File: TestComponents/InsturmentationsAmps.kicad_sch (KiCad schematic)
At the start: 42 parts, among them SW2 SW_DP3T, SW3 SW_DPDT, U3 REF200AU, U4 MCP6L01x-xLT

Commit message: SpectDrone Development
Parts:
- CS1, CS6: footprint Capacitor_SMD:C_0805_2012Metric -> Capacitor_SMD:C_0603_1608Metric; Part Number (none) -> 06035J100FBTTR
- CS2, CS3, CS7, CS8: footprint Capacitor_SMD:C_0805_2012Metric -> Capacitor_SMD:C_0402_1005Metric; Part Number (none) -> 04023J1R1PBSTR
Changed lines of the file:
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@@
       (effects (font (size 1.27 1.27)) (justify left))
     )
-    (property "Footprint" "Capacitor_SMD:C_0805_2012Metric" (id 2) (at 217.17 44.45 0)
+    (property "Footprint" "Capacitor_SMD:C_0402_1005Metric" (id 2) (at 217.17 44.45 0)
       (effects (font (size 1.27 1.27)) hide)
     )
     (property "Datasheet" "~" (id 3) (at 217.17 44.45 0)
+      (effects (font (size 1.27 1.27)) hide)
+    )
+    (property "Part Number" "04023J1R1PBSTR" (id 4) (at 217.17 44.45 0)
       (effects (font (size 1.27 1.27)) hide)
     )
@@
       (effects (font (size 1.27 1.27)) (justify left))
     )
-    (property "Footprint" "Capacitor_SMD:C_0805_2012Metric" (id 2) (at 214.63 54.61 0)
+    (property "Footprint" "Capacitor_SMD:C_0603_1608Metric" (id 2) (at 214.63 54.61 0)
       (effects (font (size 1.27 1.27)) hide)
     )
     (property "Datasheet" "~" (id 3) (at 214.63 54.61 0)
+      (effects (font (size 1.27 1.27)) hide)
+    )
+    (property "Part Number" "06035J100FBTTR" (id 4) (at 214.63 54.61 0)
       (effects (font (size 1.27 1.27)) hide)
     )
@@
       (effects (font (size 1.27 1.27)) (justify left))
     )
-    (property "Footprint" "Capacitor_SMD:C_0805_2012Metric" (id 2) (at 214.63 85.09 0)
+    (property "Footprint" "Capacitor_SMD:C_0603_1608Metric" (id 2) (at 214.63 85.09 0)
       (effects (font (size 1.27 1.27)) hide)
     )
     (property "Datasheet" "~" (id 3) (at 214.63 85.09 0)
+      (effects (font (size 1.27 1.27)) hide)
+    )
+    (property "Part Number" "06035J100FBTTR" (id 4) (at 214.63 85.09 0)
       (effects (font (size 1.27 1.27)) hide)
     )
@@
       (effects (font (size 1.27 1.27)) (justify left))
     )
-    (property "Footprint" "Capacitor_SMD:C_0805_2012Metric" (id 2) (at 214.63 95.25 0)
+    (property "Footprint" "Capacitor_SMD:C_0402_1005Metric" (id 2) (at 214.63 95.25 0)
       (effects (font (size 1.27 1.27)) hide)
     )
@@
       (effects (font (size 1.27 1.27)) hide)
     )
+    (property "Part Number" "04023J1R1PBSTR" (id 4) (at 214.63 95.25 0)
+      (effects (font (size 1.27 1.27)) hide)
+    )
     (pin "1")
     (pin "2")
@@
       (effects (font (size 1.27 1.27)) (justify left))
     )
-    (property "Footprint" "Capacitor_SMD:C_0805_2012Metric" (id 2) (at 214.63 64.77 0)
+    (property "Footprint" "Capacitor_SMD:C_0402_1005Metric" (id 2) (at 214.63 64.77 0)
       (effects (font (size 1.27 1.27)) hide)
     )
@@
       (effects (font (size 1.27 1.27)) hide)
     )
+    (property "Part Number" "04023J1R1PBSTR" (id 4) (at 214.63 64.77 0)
+      (effects (font (size 1.27 1.27)) hide)
+    )
     (pin "1")
     (pin "2")
@@
       (effects (font (size 1.27 1.27)) (justify left))
     )
-    (property "Footprint" "Capacitor_SMD:C_0805_2012Metric" (id 2) (at 217.17 74.93 0)
+    (property "Footprint" "Capacitor_SMD:C_0402_1005Metric" (id 2) (at 217.17 74.93 0)
       (effects (font (size 1.27 1.27)) hide)
     )
@@
       (effects (font (size 1.27 1.27)) hide)
     )
+    (property "Part Number" "04023J1R1PBSTR" (id 4) (at 217.17 74.93 0)
+      (effects (font (size 1.27 1.27)) hide)
+    )

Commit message: SpectDrone Development
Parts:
- CS10, CS11, CS13, CS5: Part Number (none) -> CL21B104KACNNNC
- CS12, CS4, CS9: Part Number (none) -> CL21A106KACLRNC
- JPD1, JPD2, JPD3, JPD4, JPD5, JPD6, PD1, PD2: now left out of the parts list
- R1: Part Number (none) -> ERA-6VRW1002V
- R2: Part Number (none) -> ERJ-PB6B2671V
- RS3, RS6, RS7, RS8: Part Number (none) -> ERA-6VEB3300V
- R_{C}1: Part Number (none) -> ERJ-PB6B4990V
- R_{PD.bias}1, R_{PD.bias}2: Part Number (none) -> ERJ-6GEY0R00V
- R_{PD}1, R_{PD}2: Part Number (none) -> ERA-6AEB105V
- R_{PD}1.1, R_{PD}2.1: Part Number (none) -> ERJ-6ENF2001V
- SW2: Part Number (none) -> JS203011JAQN
- SW3: Part Number (none) -> JS202011JAQN
- U3: Part Number (none) -> REF200AU
- U4: Part Number (none) -> MCP6L01T-E/LT
- US1, US2: Part Number (none) -> AD8221ARMZ
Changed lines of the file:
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@@
+      (effects (font (size 1.27 1.27)) hide)
+    )
+    (property "Part Number" "ERJ-6ENF2001V" (id 4) (at 195.58 80.01 0)
       (effects (font (size 1.27 1.27)) hide)
     )
@@
     )
     (property "Datasheet" "~" (id 3) (at 243.84 67.31 0)
+      (effects (font (size 1.27 1.27)) hide)
+    )
+    (property "Part Number" "CL21B104KACNNNC" (id 4) (at 243.84 67.31 0)
       (effects (font (size 1.27 1.27)) hide)
     )
@@
     )
     (property "Datasheet" "https://www.analog.com/media/en/technical-documentation/data-sheets/AD8236.pdf" (id 3) (at 248.92 44.45 0)
+      (effects (font (size 1.27 1.27)) hide)
+    )
+    (property "Part Number" "AD8221ARMZ" (id 4) (at 240.03 54.61 0)
       (effects (font (size 1.27 1.27)) hide)
     )
@@
       (effects (font (size 1.27 1.27)) hide)
     )
+    (property "Part Number" "ERA-6VEB3300V" (id 4) (at 208.28 59.69 0)
+      (effects (font (size 1.27 1.27)) hide)
+    )
     (pin "1")
     (pin "2")
@@
       (effects (font (size 1.27 1.27)) hide)
     )
+    (property "Part Number" "ERA-6VRW1002V" (id 4) (at 62.23 98.425 0)
+      (effects (font (size 1.27 1.27)) hide)
+    )
     (pin "1")
     (pin "2")
@@
     )
     (property "Datasheet" "~" (id 3) (at 200.025 54.61 0)
+      (effects (font (size 1.27 1.27)) hide)
+    )
+    (property "Part Number" "ERA-6AEB105V" (id 4) (at 200.025 54.61 0)
       (effects (font (size 1.27 1.27)) hide)
     )
@@
     )
     (property "Datasheet" "https://www.analog.com/media/en/technical-documentation/data-sheets/AD8236.pdf" (id 3) (at 248.92 74.93 0)
+      (effects (font (size 1.27 1.27)) hide)
+    )
+    (property "Part Number" "AD8221ARMZ" (id 4) (at 240.03 85.09 0)
       (effects (font (size 1.27 1.27)) hide)
     )
@@
       (effects (font (size 1.27 1.27)) hide)
     )
+    (property "Part Number" "ERJ-PB6B4990V" (id 4) (at 125.73 57.15 0)
+      (effects (font (size 1.27 1.27)) hide)
+    )
     (pin "1")
     (pin "2")
   )
   (symbol (lib_id "Jumper:SolderJumper_2_Bridged") (at 194.945 59.69 0) (unit 1)
-    (in_bom yes) (on_board yes)
+    (in_bom no) (on_board yes)
     (property "Reference" "JPD3" (id 0) (at 194.945 62.23 0))
     (property "Value" "SolderJumper_2_Bridged" (id 1) (at 201.295 62.23 0)
@@
     )
     (property "Datasheet" "~" (id 3) (at 208.28 90.17 0)
+      (effects (font (size 1.27 1.27)) hide)
+    )
+    (property "Part Number" "ERA-6VEB3300V" (id 4) (at 208.28 90.17 0)
       (effects (font (size 1.27 1.27)) hide)
     )
@@
     (property "Datasheet" "www.ti.com/lit/ds/symlink/ref200.pdf" (id 3) (at 64.135 71.755 0)
       (effects (font (size 1.27 1.27) italic) hide)
+    )
+    (property "Part Number" "REF200AU" (id 4) (at 71.755 71.755 0)
+      (effects (font (size 1.27 1.27)) hide)
     )
     (pin "6")
@@
       (effects (font (size 1.27 1.27)) hide)
     )
+    (property "Part Number" "JS203011JAQN" (id 4) (at 152.4 46.99 0)
+      (effects (font (size 1.27 1.27)) hide)
+    )
     (pin "1")
     (pin "2")
@@
   )
   (symbol (lib_id "Sensor_Optical:S13360-3025CS") (at 182.88 54.61 270) (unit 1)
-    (in_bom yes) (on_board yes)
+    (in_bom no) (on_board yes)
     (property "Reference" "PD1" (id 0) (at 179.07 53.34 90))
     (property "Value" "S1336-18BK" (id 1) (at 173.99 55.88 90))
@@
   )
   (symbol (lib_id "Jumper:SolderJumper_2_Bridged") (at 186.69 80.01 0) (unit 1)
-    (in_bom yes) (on_board yes)
+    (in_bom no) (on_board yes)
     (property "Reference" "JPD4" (id 0) (at 186.69 82.55 0))
     (property "Value" "SolderJumper_2_Bridged" (id 1) (at 193.04 82.55 0)
@@
       (effects (font (size 1.27 1.27) italic) hide)
     )
+    (property "Part Number" "REF200AU" (id 4) (at 68.58 52.705 0)
+      (effects (font (size 1.27 1.27)) hide)
+    )
     (pin "6")
     (pin "2")
@@
       (effects (font (size 1.27 1.27)) hide)
     )
+    (property "Part Number" "CL21A106KACLRNC" (id 4) (at 231.14 67.31 0)
+      (effects (font (size 1.27 1.27)) hide)
+    )
     (pin "1")
     (pin "2")
   )
   (symbol (lib_id "Jumper:SolderJumper_2_Bridged") (at 186.69 49.53 0) (unit 1)
-    (in_bom yes) (on_board yes)
+    (in_bom no) (on_board yes)
     (property "Reference" "JPD1" (id 0) (at 186.69 52.07 0))
     (property "Value" "SolderJumper_2_Bridged" (id 1) (at 193.04 52.07 0)
@@
       (effects (font (size 1.27 1.27)) hide)
     )
+    (property "Part Number" "CL21A106KACLRNC" (id 4) (at 50.8 114.935 0)
+      (effects (font (size 1.27 1.27)) hide)
+    )
     (pin "1")
     (pin "2")
@@
       (effects (font (size 1.27 1.27)) hide)
     )
+    (property "Part Number" "CL21B104KACNNNC" (id 4) (at 243.84 97.79 0)
+      (effects (font (size 1.27 1.27)) hide)
+    )
     (pin "1")
     (pin "2")
@@
       (effects (font (size 1.27 1.27)) hide)
     )
+    (property "Part Number" "ERJ-6ENF2001V" (id 4) (at 195.58 49.53 0)
+      (effects (font (size 1.27 1.27)) hide)
+    )
     (pin "1")
     (pin "2")
@@
       (effects (font (size 1.27 1.27)) hide)
     )
+    (property "Part Number" "CL21B104KACNNNC" (id 4) (at 41.275 114.935 0)
+      (effects (font (size 1.27 1.27)) hide)
+    )
     (pin "1")
     (pin "2")
   )
   (symbol (lib_id "Sensor_Optical:S13360-3025CS") (at 182.88 85.09 270) (unit 1)
-    (in_bom yes) (on_board yes)
+    (in_bom no) (on_board yes)
     (property "Reference" "PD2" (id 0) (at 179.07 83.82 90))
     (property "Value" "S1336-18BK" (id 1) (at 173.99 86.36 90))
@@
       (effects (font (size 1.27 1.27)) hide)
     )
+    (property "Part Number" "ERJ-6GEY0R00V" (id 4) (at 200.025 95.25 0)
+      (effects (font (size 1.27 1.27)) hide)
+    )
     (pin "1")
     (pin "2")
@@
       (effects (font (size 1.27 1.27)) hide)
     )
+    (property "Part Number" "ERJ-PB6B2671V" (id 4) (at 62.23 123.825 0)
+      (effects (font (size 1.27 1.27)) hide)
+    )
     (pin "1")
     (pin "2")
@@
     )
     (property "Datasheet" "~" (id 3) (at 208.28 80.01 0)
+      (effects (font (size 1.27 1.27)) hide)
+    )
+    (property "Part Number" "ERA-6VEB3300V" (id 4) (at 208.28 80.01 0)
       (effects (font (size 1.27 1.27)) hide)
     )
@@
       (effects (font (size 1.27 1.27)) hide)
     )
+    (property "Part Number" "CL21A106KACLRNC" (id 4) (at 231.14 97.79 0)
+      (effects (font (size 1.27 1.27)) hide)
+    )
     (pin "1")
     (pin "2")
@@
       (effects (font (size 1.27 1.27)) hide)
     )
+    (property "Part Number" "ERA-6AEB105V" (id 4) (at 200.025 85.09 0)
+      (effects (font (size 1.27 1.27)) hide)
+    )
     (pin "1")
     (pin "2")
   )
   (symbol (lib_id "Jumper:SolderJumper_2_Open") (at 190.5 54.61 90) (unit 1)
-    (in_bom yes) (on_board yes)
+    (in_bom no) (on_board yes)
     (property "Reference" "JPD2" (id 0) (at 193.04 52.07 0)
       (effects (font (size 1.27 1.27)) (justify right))
@@
     )
     (property "Datasheet" "~" (id 3) (at 57.785 93.98 0)
+      (effects (font (size 1.27 1.27)) hide)
+    )
+    (property "Part Number" "CL21B104KACNNNC" (id 4) (at 57.785 93.98 0)
       (effects (font (size 1.27 1.27)) hide)
     )
@@
       (effects (font (size 1.27 1.27)) hide)
     )
+    (property "Part Number" "JS202011JAQN" (id 4) (at 115.57 57.15 0)
+      (effects (font (size 1.27 1.27)) hide)
+    )
     (pin "4")
     (pin "5")
@@
     )
     (property "Datasheet" "~" (id 3) (at 136.525 52.705 0)
+      (effects (font (size 1.27 1.27)) hide)
+    )
+    (property "Part Number" "JS203011JAQN" (id 4) (at 152.4 57.15 0)
       (effects (font (size 1.27 1.27)) hide)
     )
@@
       (effects (font (size 1.27 1.27)) hide)
     )
+    (property "Part Number" "JS202011JAQN" (id 4) (at 115.57 46.99 0)
+      (effects (font (size 1.27 1.27)) hide)
+    )
     (pin "1")
     (pin "2")
@@
       (effects (font (size 1.27 1.27) italic) hide)
     )
+    (property "Part Number" "REF200AU" (id 4) (at 74.93 52.705 0)
+      (effects (font (size 1.27 1.27)) hide)
+    )
     (pin "6")
     (pin "1")
@@
       (effects (font (size 1.27 1.27)) hide)
     )
+    (property "Part Number" "ERA-6VEB3300V" (id 4) (at 208.28 49.53 0)
+      (effects (font (size 1.27 1.27)) hide)
+    )
     (pin "1")
     (pin "2")
   )
   (symbol (lib_id "Jumper:SolderJumper_2_Open") (at 190.5 85.09 90) (unit 1)
-    (in_bom yes) (on_board yes)
+    (in_bom no) (on_board yes)
     (property "Reference" "JPD5" (id 0) (at 193.04 82.55 0)
       (effects (font (size 1.27 1.27)) (justify right))
@@
     )
     (property "Datasheet" "~" (id 3) (at 200.025 64.77 0)
+      (effects (font (size 1.27 1.27)) hide)
+    )
+    (property "Part Number" "ERJ-6GEY0R00V" (id 4) (at 200.025 64.77 0)
       (effects (font (size 1.27 1.27)) hide)
     )
@@
       (effects (font (size 1.27 1.27)) hide)
     )
+    (property "Part Number" "MCP6L01T-E/LT" (id 4) (at 63.5 111.125 0)
+      (effects (font (size 1.27 1.27)) hide)
+    )
     (pin "2")
     (pin "5")
@@
   )
   (symbol (lib_id "Jumper:SolderJumper_2_Bridged") (at 194.945 90.17 0) (unit 1)
-    (in_bom yes) (on_board yes)
+    (in_bom no) (on_board yes)
     (property "Reference" "JPD6" (id 0) (at 194.945 92.71 0))
     (property "Value" "SolderJumper_2_Bridged" (id 1) (at 201.295 92.71 0)

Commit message: SpectDrone Development
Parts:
- RS2, RS5: now left out of the parts list
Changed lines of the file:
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@@
   )
   (symbol (lib_id "Device:R") (at 225.425 54.61 0) (unit 1)
-    (in_bom yes) (on_board yes)
+    (in_bom no) (on_board yes)
     (property "Reference" "RS2" (id 0) (at 226.695 53.34 0)
       (effects (font (size 1.27 1.27)) (justify left))
@@
   )
   (symbol (lib_id "Device:R") (at 225.425 85.09 0) (unit 1)
-    (in_bom yes) (on_board yes)
+    (in_bom no) (on_board yes)
     (property "Reference" "RS5" (id 0) (at 226.695 83.82 0)
       (effects (font (size 1.27 1.27)) (justify left))

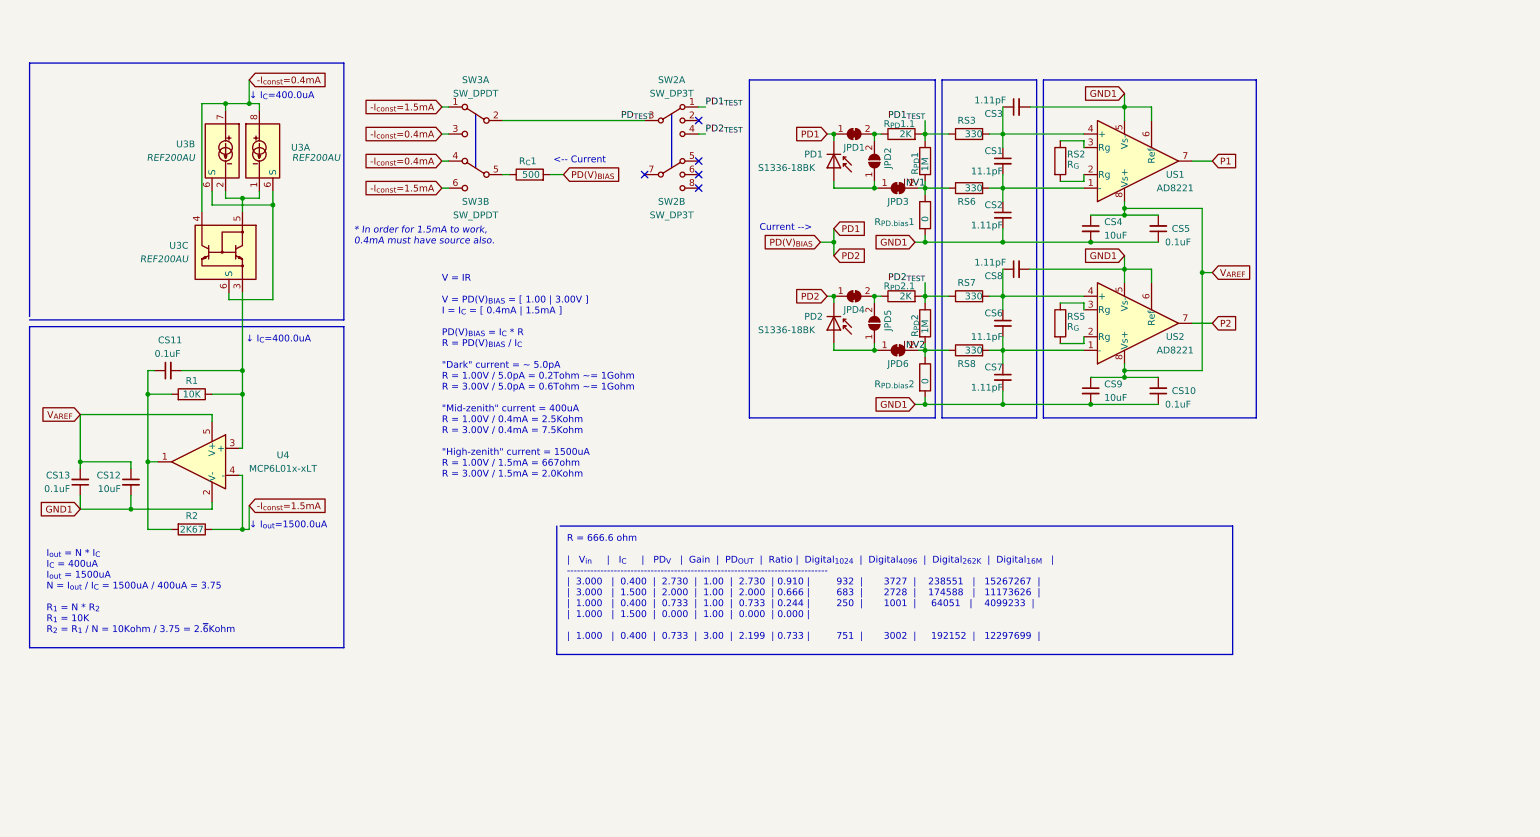
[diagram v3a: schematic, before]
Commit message: SpectDrone Development
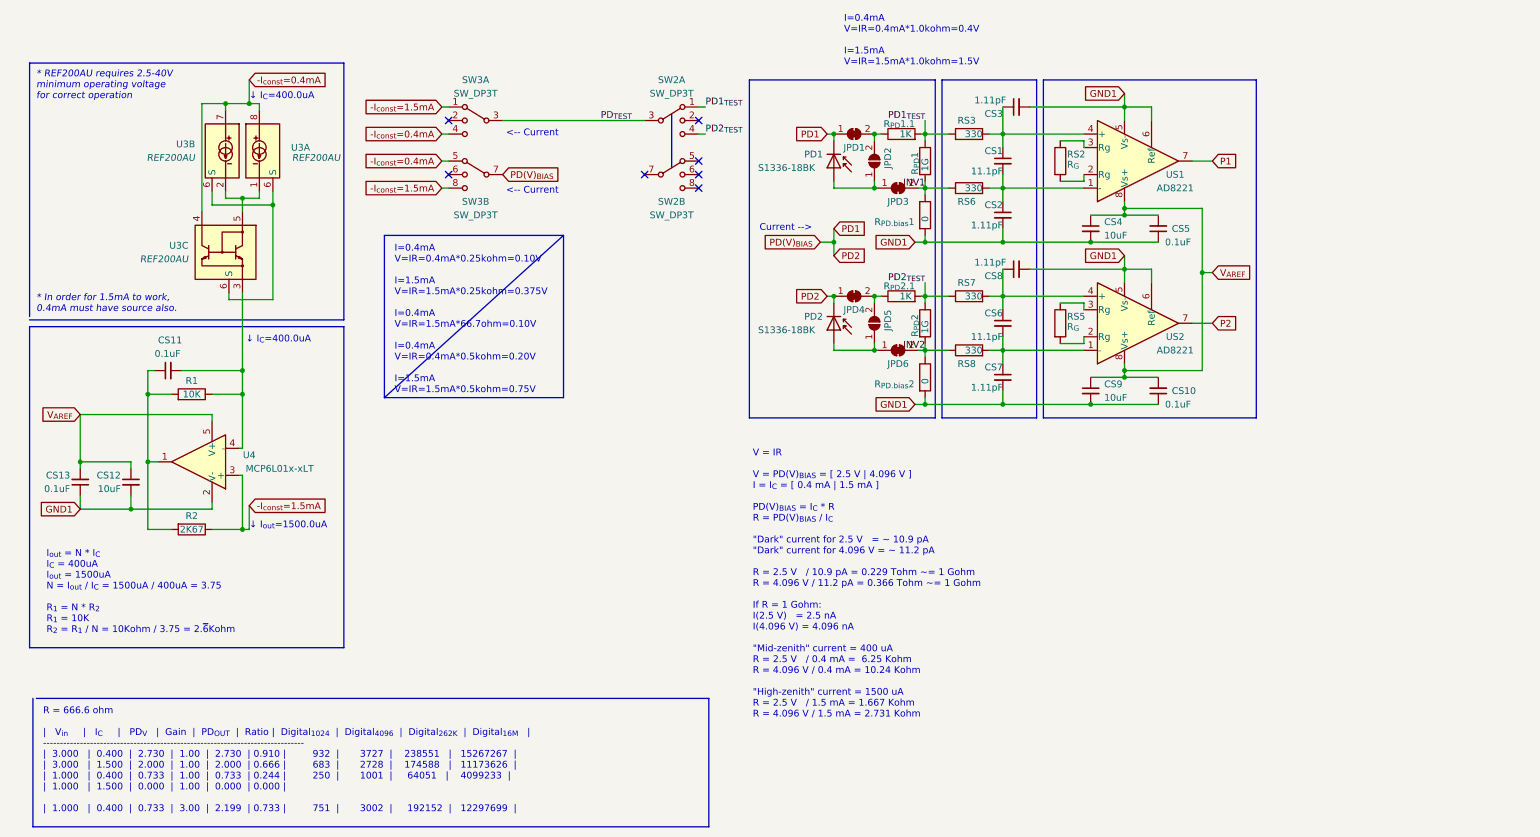
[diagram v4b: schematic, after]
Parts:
- removed R_{C}1: 500, Resistor_SMD:R_0805_2012Metric, symbol Device:R
- removed SW3: SW_DPDT, Gardenuino Custom:SW_DPDT_CK_JS202011JAQN, symbol Switch:SW_DPDT_x2
- added SW3: SW_DP3T, Gardenuino Custom:SW_DP3T_CK_JS203011JAQN, symbol Switch:SW_DP3T
- R_{PD}1, R_{PD}2: value 1M -> 1G; Part Number ERA-6AEB105V -> HVC0805Z1007JET
- R_{PD}1.1, R_{PD}2.1: value 2K -> 1K; Part Number ERJ-6ENF2001V -> (none)
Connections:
- net -I_{const}=0.4mA: now also SW3.4, SW3.5
- net -I_{const}=1.5mA: now also U4.3 (+), SW3.1, SW3.8; no longer U4.4 (-)
- net PD(V)_{BIAS}: now also SW3.7
- net PD_{TEST}: now also SW3.3
- net at CS11.2, R1.1, U3.3: now also U4.4 (-); no longer U4.3 (+)
- no-connect marks 5 -> 7
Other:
- note added: "* REF200AU requires 2.5-40V minimum operating voltage for correct operation"
- note added: "I=0.4mA V=IR=0.4mA*0.25kohm=0.10V I=1.5mA V=IR=1.5mA*0.25kohm=0.375V I=0.4mA V=IR=1.5mA*66.7ohm=0.10V I=0.4mA V=IR=0.4mA*0.5kohm=0.20V I=1.5mA V=IR=1.5mA*0.5kohm=0.75V"
- note added: "I=0.4mA V=IR=0.4mA*1.0kohm=0.4V I=1.5mA V=IR=1.5mA*1.0kohm=1.5V"
- note added: "V = IR V = PD(V)_{BIAS} = [ 2.5 V | 4.096 V ] I = I_{C} = [ 0.4 mA | 1.5 mA ] PD(V)_{BIAS} = I_{C} * R R = PD(V)_{BIAS} / I_{C} "Dark" current for 2.5 V = ~ 10.9 pA "Dark" current for 4.096 V = ~ 11.2 pA R = 2.5 V / 10.9 pA = 0.229 Tohm ~= 1 Gohm R = 4.096 V / 11.2 pA = 0.366 Tohm ~= 1 Gohm If R = 1 Gohm: I(2.5 V) = 2.5 nA I(4.096 V) = 4.096 nA "Mid-zenith" current = 400 uA R = 2.5 V / 0.4 mA = 6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"
- note removed: "V = IR V = PD(V)_{BIAS} = [ 1.00 | 3.00V ] I = I_{C} = [ 0.4mA | 1.5mA ] PD(V)_{BIAS} = I_{C} * R R = PD(V)_{BIAS} / I_{C} "Dark" current = ~ 5.0pA R = 1.00V / 5.0pA = 0.2Tohm ~= 1Gohm R = 3.00V / 5.0pA = 0.6Tohm ~= 1Gohm "Mid-zenith" current = 400uA R = 1.00V / 0.4mA = 2.5Kohm R = 3.00V / 0.4mA = 7.5Kohm "High-zenith" current = 1500uA R = 1.00V / 1.5mA = 667ohm R = 3.00V / 1.5mA = 2.0Kohm"
- moved on the sheet: U4
